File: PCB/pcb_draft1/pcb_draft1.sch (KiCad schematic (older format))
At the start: 50 parts

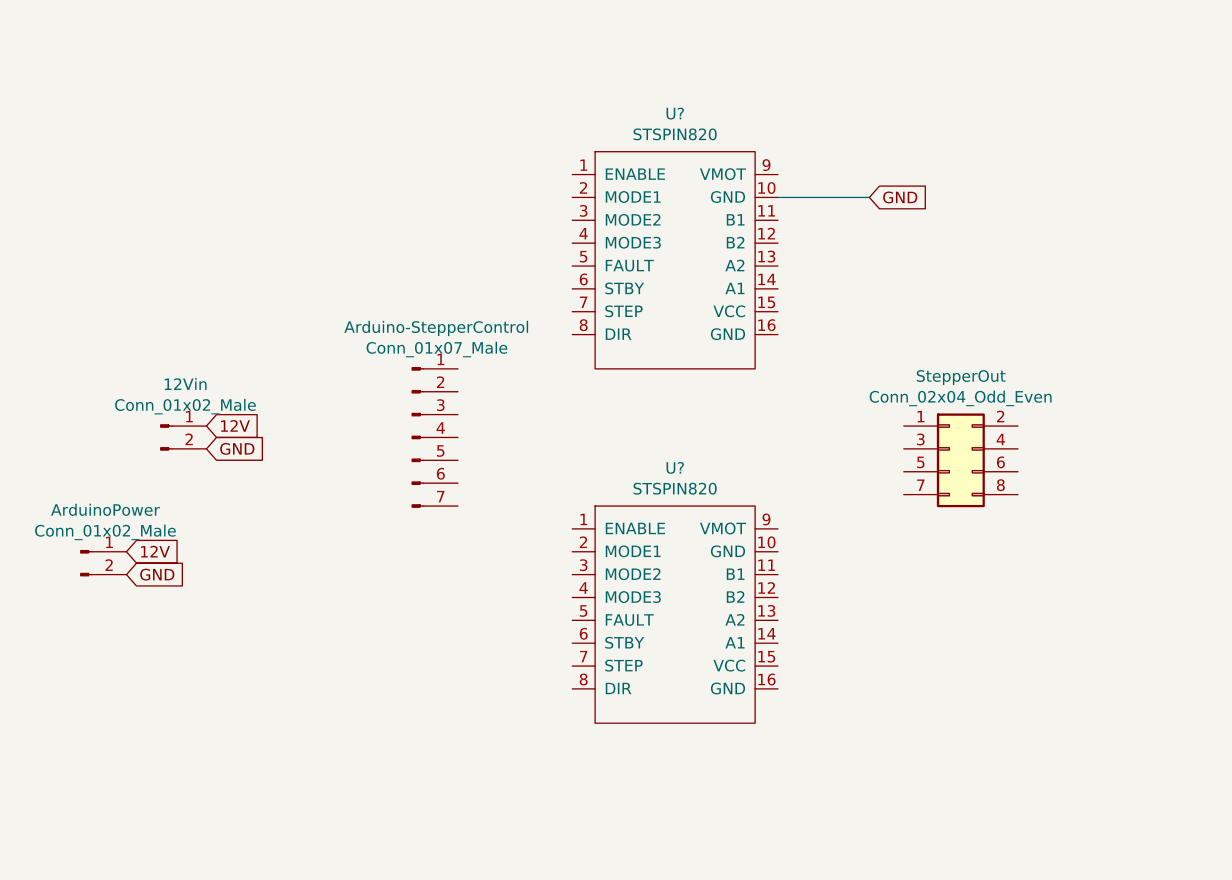
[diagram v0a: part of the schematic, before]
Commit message: Finish wiring for PCB First Draft
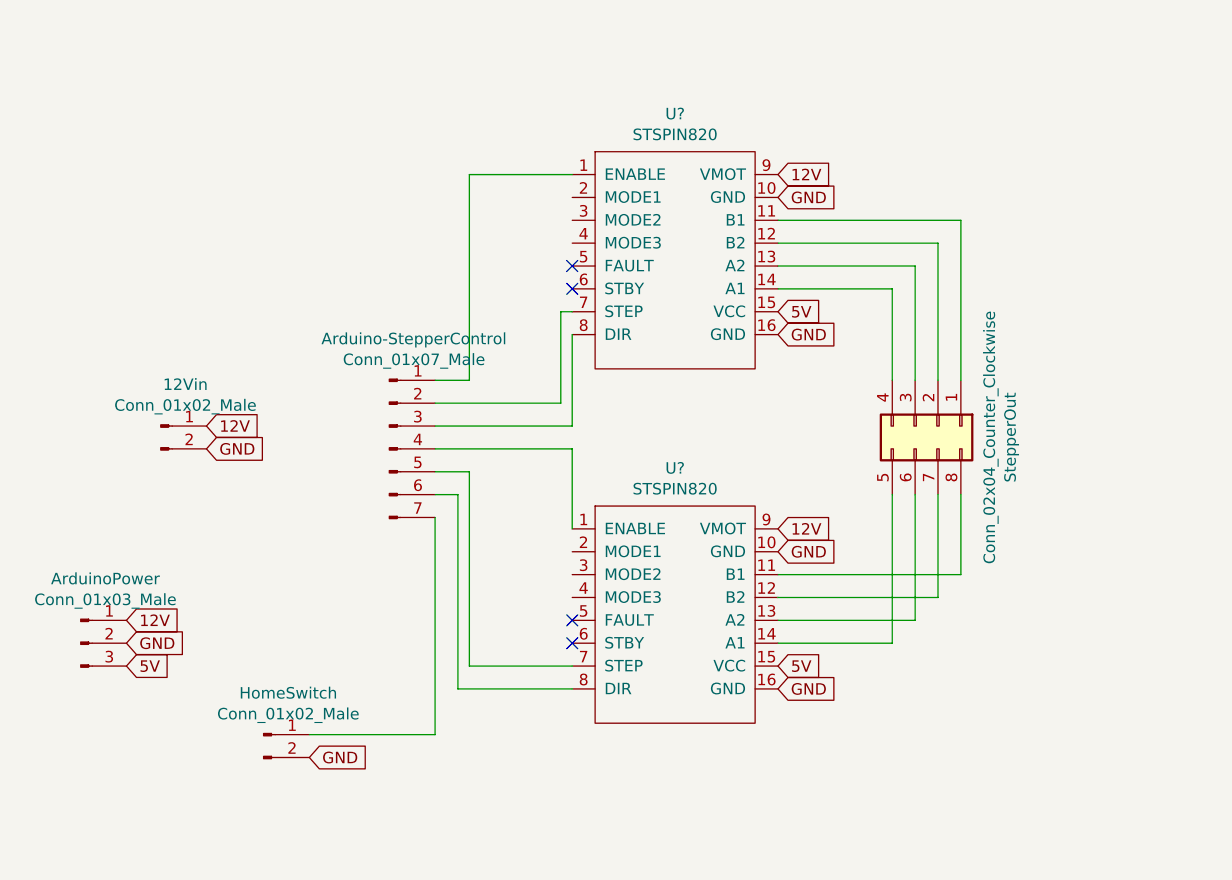
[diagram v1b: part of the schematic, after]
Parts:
- removed ArduinoPower: Conn_01x02_Male, symbol Connector:Conn_01x02_Male
- removed StepperOut: Conn_02x04_Odd_Even, symbol Connector_Generic:Conn_02x04_Odd_Even
- added ArduinoPower: Conn_01x03_Male, symbol Connector:Conn_01x03_Male
- added HomeSwitch: Conn_01x02_Male, symbol Connector:Conn_01x02_Male
- added StepperOut: Conn_02x04_Counter_Clockwise, symbol Connector_Generic:Conn_02x04_Counter_Clockwise
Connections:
- net 12V: now also U?.9 (VMOT), U?.9 (VMOT), ArduinoPower.1 (Pin_1)
- net GND: now also U?.10 (GND), U?.16 (GND), U?.16 (GND), ArduinoPower.2 (Pin_2), HomeSwitch.2 (Pin_2)
- net at Arduino-StepperControl.1 (Pin_1): now also U?.1 (ENABLE)
- net at Arduino-StepperControl.2 (Pin_2): now also U?.7 (STEP)
- net at Arduino-StepperControl.3 (Pin_3): now also U?.8 (DIR)
- net at Arduino-StepperControl.4 (Pin_4): now also U?.1 (ENABLE)
- net at Arduino-StepperControl.5 (Pin_5): now also U?.7 (STEP)
- net at Arduino-StepperControl.6 (Pin_6): now also U?.8 (DIR)
- net at Arduino-StepperControl.7 (Pin_7): now also HomeSwitch.1 (Pin_1)
- net at U?.11 (B1): now also StepperOut.8 (Pin_8)
- net at U?.12 (B2): now also StepperOut.7 (Pin_7)
- net at U?.13 (A2): now also StepperOut.6 (Pin_6)
- net at U?.14 (A1): now also StepperOut.5 (Pin_5)
- net 5V: now reaches U?.15 (VCC)
- net 5V: now also U?.15 (VCC), ArduinoPower.3 (Pin_3)
- net at U?.11 (B1): now also StepperOut.1 (Pin_1)
- net at U?.12 (B2): now also StepperOut.2 (Pin_2)
- net at U?.13 (A2): now also StepperOut.3 (Pin_3)
- net at U?.14 (A1): now also StepperOut.4 (Pin_4)
- no-connect marks 0 -> 4
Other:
- moved on the sheet: Arduino-StepperControl
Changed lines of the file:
@@
 L Connector:Conn_01x07_Male Arduino-StepperControl
 U 1 1 5DB9AA25
-P 2200 5700
-F 0 "Arduino-StepperControl" H 2308 6181 50  0000 C CNN
-F 1 "Conn_01x07_Male" H 2308 6090 50  0000 C CNN
-F 2 "" H 2200 5700 50  0001 C CNN
-F 3 "~" H 2200 5700 50  0001 C CNN
-	1    2200 5700
-	1    0    0    -1
-$EndComp
-$Comp
-L Connector_Generic:Conn_02x04_Odd_Even StepperOut
-U 1 1 5DB9C5BF
-P 4550 5750
-F 0 "StepperOut" H 4600 6067 50  0000 C CNN
-F 1 "Conn_02x04_Odd_Even" H 4600 5976 50  0000 C CNN
-F 2 "" H 4550 5750 50  0001 C CNN
-F 3 "~" H 4550 5750 50  0001 C CNN
-	1    4550 5750
+P 2100 5750
+F 0 "Arduino-StepperControl" H 2208 6231 50  0000 C CNN
+F 1 "Conn_01x07_Male" H 2208 6140 50  0000 C CNN
+F 2 "" H 2100 5750 50  0001 C CNN
+F 3 "~" H 2100 5750 50  0001 C CNN
+	1    2100 5750
 	1    0    0    -1
 $EndComp
@@
 $EndComp
 $Comp
-L Connector:Conn_01x02_Male ArduinoPower
-U 1 1 5DB9F6C1
-P 750 6200
-F 0 "ArduinoPower" H 858 6381 50  0000 C CNN
-F 1 "Conn_01x02_Male" H 858 6290 50  0000 C CNN
-F 2 "" H 750 6200 50  0001 C CNN
-F 3 "~" H 750 6200 50  0001 C CNN
-	1    750  6200
-	1    0    0    -1
-$EndComp
-$Comp
 L CustomSymbols:STSPIN820 U?
 U 1 1 5DBB0CCE
@@
 	1    0    0    -1
 $EndComp
-Text GLabel 4200 4650 2    50   Input ~ 0
-GND
-Wire Wire Line
-	3800 4650 4200 4650
+Text GLabel 3800 4650 2    50   Input ~ 0
+GND
 Text GLabel 11100 4050 2    50   Input ~ 0
 12V
@@
 Text GLabel 1300 5750 2    50   Input ~ 0
 GND
-Text GLabel 950  6200 2    50   Input ~ 0
-12V
-Text GLabel 950  6300 2    50   Input ~ 0
+Text GLabel 950  6500 2    50   Input ~ 0
+12V
+Text GLabel 950  6600 2    50   Input ~ 0
 GND
 Text GLabel 8850 600  0    50   Input ~ 0
@@
 Wire Wire Line
 	10950 3950 10950 4050
+Text GLabel 3800 6800 2    50   Input ~ 0
+GND
+Text GLabel 3800 6200 2    50   Input ~ 0
+GND
+Text GLabel 3800 5250 2    50   Input ~ 0
+GND
+Text GLabel 3800 5150 2    50   Input ~ 0
+5V
+Text GLabel 3800 6700 2    50   Input ~ 0
+5V
+$Comp
+L Connector:Conn_01x03_Male ArduinoPower
+U 1 1 5DD3A23F
+P 750 6600
+F 0 "ArduinoPower" H 858 6881 50  0000 C CNN
+F 1 "Conn_01x03_Male" H 858 6790 50  0000 C CNN
+F 2 "" H 750 6600 50  0001 C CNN
+F 3 "~" H 750 6600 50  0001 C CNN
+	1    750  6600
+	1    0    0    -1
+$EndComp
+Text GLabel 950  6700 2    50   Input ~ 0
+5V
+Text GLabel 3800 4550 2    50   Input ~ 0
+12V
+Text GLabel 3800 6100 2    50   Input ~ 0
+12V
+$Comp
+L Connector_Generic:Conn_02x04_Counter_Clockwise StepperOut
+U 1 1 5DD4CD3C
+P 4500 5650
+F 0 "StepperOut" H 4550 5967 50  0000 C CNN
+F 1 "Conn_02x04_Counter_Clockwise" H 4550 5876 50  0000 C CNN
+F 2 "" H 4500 5650 50  0001 C CNN
+F 3 "~" H 4500 5650 50  0001 C CNN
+	1    4500 5650
+	0    1    1    0
+$EndComp
+Wire Wire Line
+	3800 4750 4600 4750
+Wire Wire Line
+	4600 4750 4600 5450
+Wire Wire Line
+	3800 4850 4500 4850
+Wire Wire Line
+	4500 4850 4500 5450
+Wire Wire Line
+	3800 4950 4400 4950
+Wire Wire Line
+	4400 4950 4400 5450
+Wire Wire Line
+	3800 5050 4300 5050
+Wire Wire Line
+	4300 5050 4300 5450
+Wire Wire Line
+	3800 6600 4300 6600
+Wire Wire Line
+	4300 6600 4300 5950
+Wire Wire Line
+	3800 6500 4400 6500
+Wire Wire Line
+	4400 6500 4400 5950
+Wire Wire Line
+	3800 6400 4500 6400
+Wire Wire Line
+	4500 6400 4500 5950
+Wire Wire Line
+	3800 6300 4600 6300
+Wire Wire Line
+	4600 6300 4600 5950
+Wire Wire Line
+	2300 5650 2900 5650
+Wire Wire Line
+	2900 5650 2900 5250
+Wire Wire Line
+	2300 5550 2850 5550
+Wire Wire Line
+	2850 5550 2850 5150
+Wire Wire Line
+	2850 5150 2900 5150
+Wire Wire Line
+	2300 5450 2450 5450
+Wire Wire Line
+	2450 5450 2450 4550
+Wire Wire Line
+	2450 4550 2900 4550
+NoConn ~ 2900 4950
+NoConn ~ 2900 5050
+NoConn ~ 2900 6500
+NoConn ~ 2900 6600
+Wire Wire Line
+	2300 5750 2900 5750
+Wire Wire Line
+	2900 5750 2900 6100
+Wire Wire Line
+	2300 5850 2450 5850
+Wire Wire Line
+	2450 5850 2450 6700
+Wire Wire Line
+	2450 6700 2900 6700
+Wire Wire Line
+	2300 5950 2400 5950
+Wire Wire Line
+	2400 5950 2400 6800
+Wire Wire Line
+	2400 6800 2900 6800
+$Comp
+L Connector:Conn_01x02_Male HomeSwitch
+U 1 1 5DDC4700
+P 1550 7000
+F 0 "HomeSwitch" H 1658 7181 50  0000 C CNN
+F 1 "Conn_01x02_Male" H 1658 7090 50  0000 C CNN
+F 2 "" H 1550 7000 50  0001 C CNN
+F 3 "~" H 1550 7000 50  0001 C CNN
+	1    1550 7000
+	1    0    0    -1
+$EndComp
+Wire Wire Line
+	1750 7000 2300 7000
+Wire Wire Line
+	2300 7000 2300 6050
+Text GLabel 1750 7100 2    50   Input ~ 0
+GND
 $EndSCHEMATC
